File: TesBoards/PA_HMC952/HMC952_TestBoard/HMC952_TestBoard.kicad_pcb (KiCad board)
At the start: 2 copper layers, 70 x 45 mm, 30 parts, among them J1 SMA, J2 SMA, J3 VDD, J4 VGG, J5 VDET, U1 HMC952ALP5GE

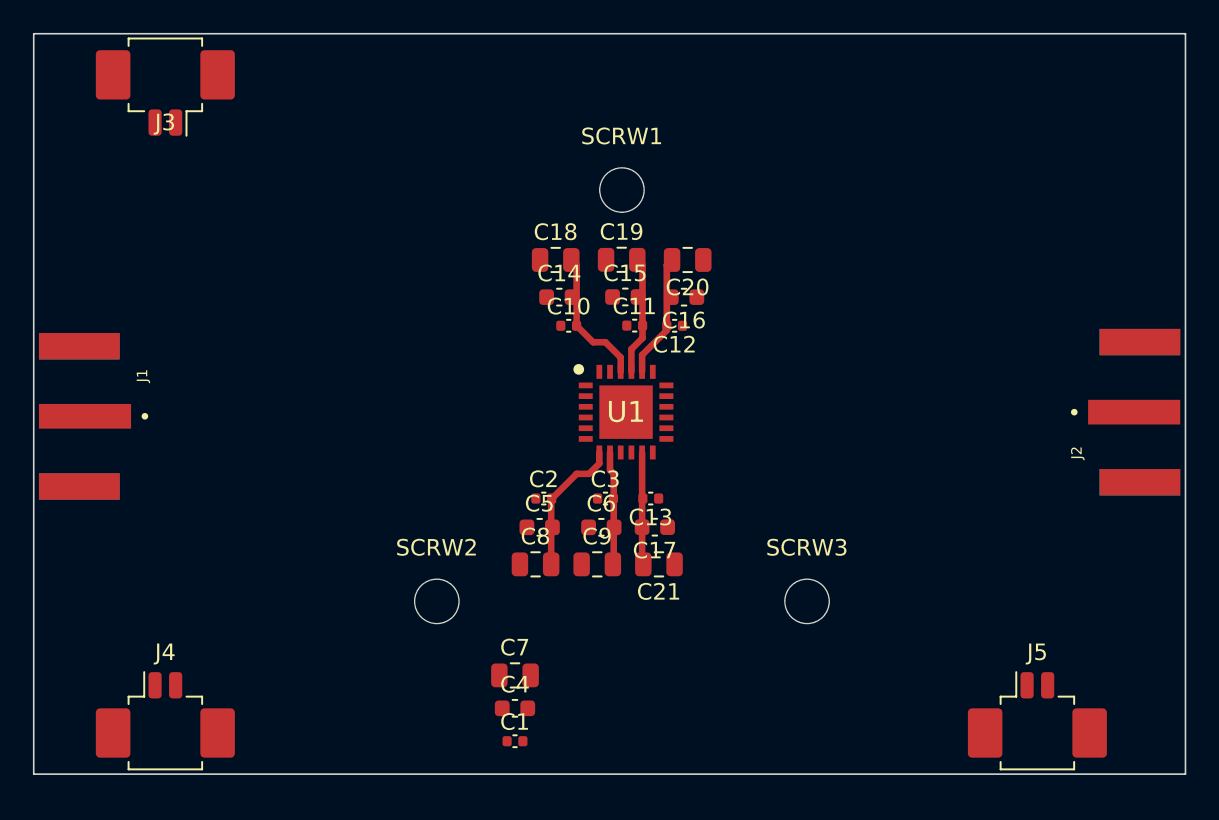
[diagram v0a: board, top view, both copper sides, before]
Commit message: PA TB
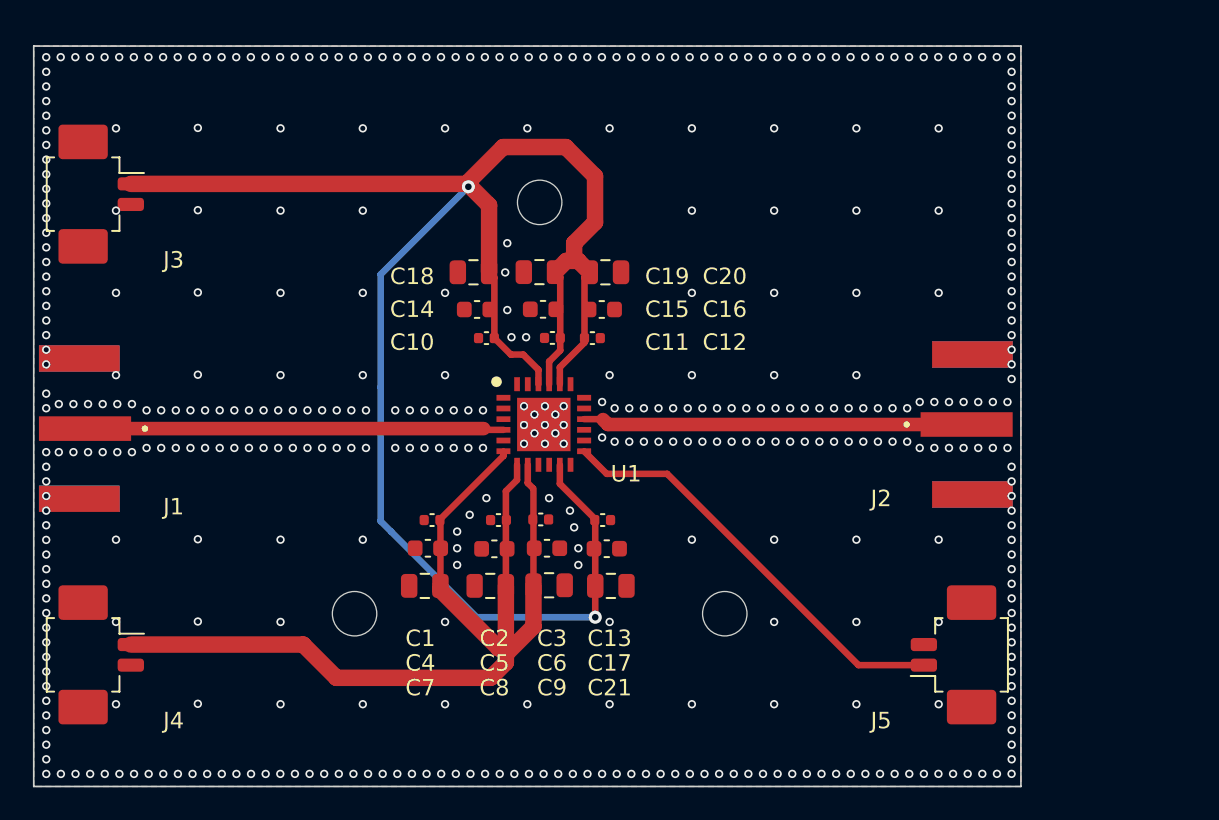
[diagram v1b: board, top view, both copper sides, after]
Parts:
- moved C1 14.4 mm to (130.2, 98.8)
- moved C4 11.1 mm to (130.0, 100.5)
- moved J2 10.2 mm to (165.5, 93.0)
- moved J3 8.11 mm to (109.5, 79.0), turned to -90 degrees
- moved C7 7.72 mm to (129.8, 102.8)
- moved J4 6.19 mm to (109.5, 107.0), turned to -90 degrees
- moved J5 6.19 mm to (162.5, 107.0), turned to 90 degrees
- moved C10 5.06 mm to (133.5, 87.8)
- moved C11 5.06 mm to (137.5, 87.7)
- moved C12 5.06 mm to (140.0, 87.8)
- moved C14 5.06 mm to (132.9, 86.0)
- moved C15 5.06 mm to (137.0, 86.0)
- moved C16 5.06 mm to (140.5, 86.0)
- moved C18 5.06 mm to (132.7, 83.8)
- moved C19 5.06 mm to (136.7, 83.7)
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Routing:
- net /Vd_PA: track 30.2 -> 115.3 mm, vias 0 -> 2
- net /Vg_PA: track 15.5 -> 64.0 mm
- net /Vdet: track 0.00 -> 26.0 mm
- net /RF_In: track 0.00 -> 25.5 mm
- net /RF_out: track 0.00 -> 22.9 mm
- net GND: vias 0 -> 430
- added copper zone on B.Cu, net GND
- added copper zone on F.Cu, net GND
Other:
- board size 70 x 45 mm -> 60 x 45 mm
- board text added: "ROGERS 4350B Layers = 2 Metalization = 35 um Thinkness = 0.813 mm (32 mils) Er = 3.66 tand = 0.0037"
